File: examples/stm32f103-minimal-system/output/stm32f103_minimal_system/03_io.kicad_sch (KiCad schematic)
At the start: 3 parts, among them J2 SWD-4P

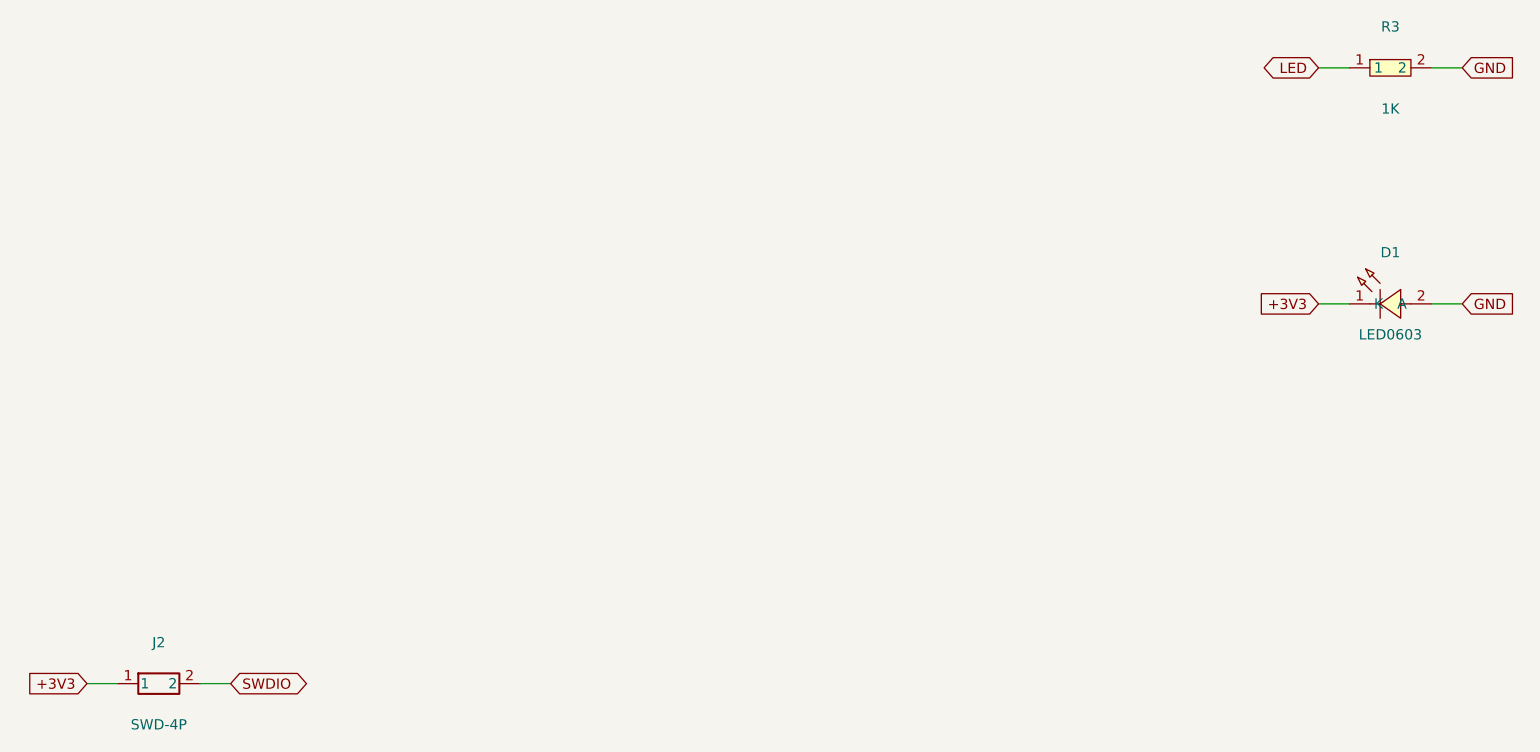
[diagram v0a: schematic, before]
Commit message: docs: refresh verified examples / 文档：刷新已验证示例
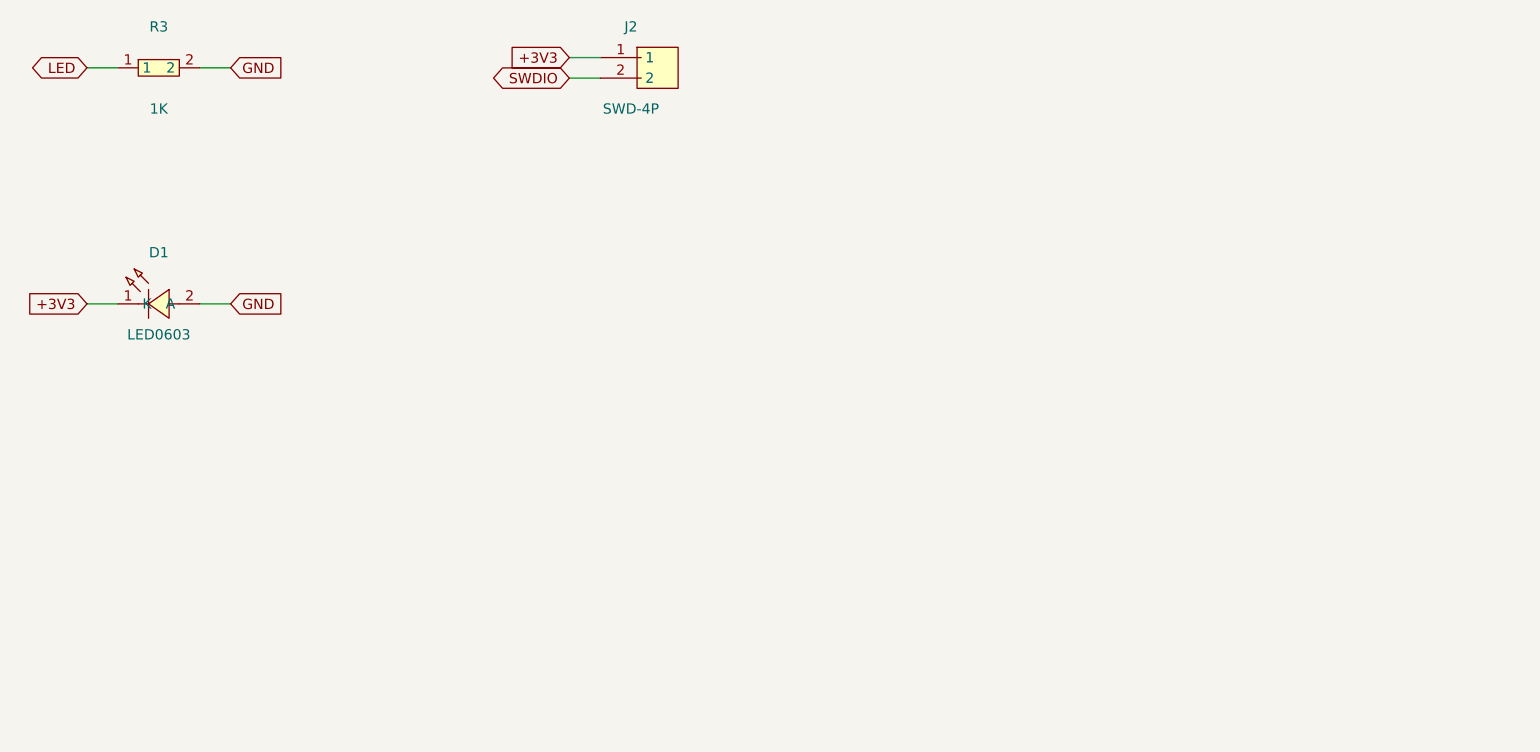
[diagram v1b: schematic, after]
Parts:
- removed J2: SWD-4P, symbol JLC-MCP:2.54mm_1_2P
- added J2: SWD-4P, JLC-MCP:HDR-TH_2P-P2.54-V-M, symbol JLC-MCP:2.54mm1_2P
- D1: footprint (none) -> JLC-MCP:LED-SMD_L1.6-W0.8-RD_GREEN-1
- R3: footprint (none) -> JLC-MCP:R0603
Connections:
- net +3V3: now also J2.1
- net SWDIO: now also J2.2
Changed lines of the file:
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@@
   (symbol
     (lib_id "JLC-MCP:RC0603JR-071KL")
-    (at 203.2 50.8 0)
+    (at 50.8 50.8 0)
     (unit 1)
     (exclude_from_sim no)
@@
     (on_board yes)
     (dnp no)
-    (property "Reference" "R3" (at 203.2 45.72 0)
+    (property "Reference" "R3" (at 50.8 45.72 0)
       (effects (font (size 1.27 1.27)))
     )
-    (property "Value" "1K" (at 203.2 55.88 0)
+    (property "Value" "1K" (at 50.8 55.88 0)
       (effects (font (size 1.27 1.27)))
     )
-    (property "Footprint" "" (at 203.2 50.8 0)
+    (property "Footprint" "JLC-MCP:R0603" (at 50.8 50.8 0)
       (hide yes)
       (effects (font (size 1.27 1.27)))
@@
     (instances
       (project "stm32f103_minimal_system"
-        (path "/9ec7504e-3b71-4439-aa58-3a2830d4ea29"
+        (path "/c5b79de1-e00a-4af4-a1c5-793330a97c08"
           (reference "R3")
           (unit 1)
@@
   (symbol
     (lib_id "JLC-MCP:APHD1608LCGCK")
-    (at 203.2 78.74 0)
+    (at 50.8 78.74 0)
     (unit 1)
     (exclude_from_sim no)
@@
     (on_board yes)
     (dnp no)
-    (property "Reference" "D1" (at 203.2 73.66 0)
+    (property "Reference" "D1" (at 50.8 73.66 0)
       (effects (font (size 1.27 1.27)))
     )
-    (property "Value" "LED0603" (at 203.2 83.82 0)
+    (property "Value" "LED0603" (at 50.8 83.82 0)
       (effects (font (size 1.27 1.27)))
     )
-    (property "Footprint" "" (at 203.2 78.74 0)
+    (property "Footprint" "JLC-MCP:LED-SMD_L1.6-W0.8-RD_GREEN-1" (at 50.8 78.74 0)
       (hide yes)
       (effects (font (size 1.27 1.27)))
@@
     (instances
       (project "stm32f103_minimal_system"
-        (path "/9ec7504e-3b71-4439-aa58-3a2830d4ea29"
+        (path "/c5b79de1-e00a-4af4-a1c5-793330a97c08"
           (reference "D1")
           (unit 1)
@@
   )
   (symbol
-    (lib_id "JLC-MCP:2.54mm_1_2P")
-    (at 50.8 127 0)
+    (lib_id "JLC-MCP:2.54mm1_2P")
+    (at 109.22 50.8 0)
     (unit 1)
     (exclude_from_sim no)
@@
     (on_board yes)
     (dnp no)
-    (property "Reference" "J2" (at 50.8 121.92 0)
+    (property "Reference" "J2" (at 109.22 45.72 0)
       (effects (font (size 1.27 1.27)))
     )
-    (property "Value" "SWD-4P" (at 50.8 132.08 0)
+    (property "Value" "SWD-4P" (at 109.22 55.88 0)
       (effects (font (size 1.27 1.27)))
     )
-    (property "Footprint" "" (at 50.8 127 0)
+    (property "Footprint" "JLC-MCP:HDR-TH_2P-P2.54-V-M" (at 109.22 50.8 0)
       (hide yes)
       (effects (font (size 1.27 1.27)))
@@
     (instances
       (project "stm32f103_minimal_system"
-        (path "/9ec7504e-3b71-4439-aa58-3a2830d4ea29"
+        (path "/c5b79de1-e00a-4af4-a1c5-793330a97c08"
           (reference "J2")
           (unit 1)
@@
     )
   )
-  (wire (pts (xy 198.12 50.8) (xy 194.31 50.8))
+  (wire (pts (xy 45.72 50.8) (xy 41.91 50.8))
     (stroke (width 0) (type default))
   )
-  (global_label "LED" (shape bidirectional) (at 194.31 50.8 0)
+  (global_label "LED" (shape bidirectional) (at 41.91 50.8 0)
     (effects (font (size 1.27 1.27)) (justify right))
   )
-  (wire (pts (xy 208.28 50.8) (xy 212.09 50.8))
+  (wire (pts (xy 55.88 50.8) (xy 59.69 50.8))
     (stroke (width 0) (type default))
   )
-  (global_label "GND" (shape input) (at 212.09 50.8 0)
+  (global_label "GND" (shape input) (at 59.69 50.8 0)
     (effects (font (size 1.27 1.27)) (justify left))
   )
-  (wire (pts (xy 198.12 80.01) (xy 194.31 80.01))
+  (wire (pts (xy 45.72 80.01) (xy 41.91 80.01))
     (stroke (width 0) (type default))
   )
-  (global_label "+3V3" (shape input) (at 194.31 80.01 0)
+  (global_label "+3V3" (shape input) (at 41.91 80.01 0)
     (effects (font (size 1.27 1.27)) (justify right))
   )
-  (wire (pts (xy 208.28 80.01) (xy 212.09 80.01))
+  (wire (pts (xy 55.88 80.01) (xy 59.69 80.01))
     (stroke (width 0) (type default))
   )
-  (global_label "GND" (shape input) (at 212.09 80.01 0)
+  (global_label "GND" (shape input) (at 59.69 80.01 0)
     (effects (font (size 1.27 1.27)) (justify left))
   )
-  (wire (pts (xy 45.72 127) (xy 41.91 127))
+  (wire (pts (xy 105.41 49.53) (xy 101.6 49.53))
     (stroke (width 0) (type default))
   )
-  (global_label "+3V3" (shape input) (at 41.91 127 0)
+  (global_label "+3V3" (shape input) (at 101.6 49.53 0)
     (effects (font (size 1.27 1.27)) (justify right))
   )
-  (wire (pts (xy 55.88 127) (xy 59.69 127))
+  (wire (pts (xy 105.41 52.07) (xy 101.6 52.07))
     (stroke (width 0) (type default))
   )
-  (global_label "SWDIO" (shape bidirectional) (at 59.69 127 0)
-    (effects (font (size 1.27 1.27)) (justify left))
+  (global_label "SWDIO" (shape bidirectional) (at 101.6 52.07 0)
+    (effects (font (size 1.27 1.27)) (justify right))
   )
   (sheet_instances
     (path "/" (page "1"))
-    (path "/fdb53bd6-e26e-42bb-8ab7-eefcb09b6f3b" (page "2"))
-    (path "/b2a7a2b2-bc8c-4209-a7e6-5e88bfab0a16" (page "3"))
-    (path "/9ec7504e-3b71-4439-aa58-3a2830d4ea29" (page "4"))
+    (path "/0219bda3-e559-4fee-b1f9-0b2f1465a67d" (page "2"))
+    (path "/da0710c1-d244-4808-8bdb-104a876a3754" (page "3"))
+    (path "/c5b79de1-e00a-4af4-a1c5-793330a97c08" (page "4"))
   )
 )
